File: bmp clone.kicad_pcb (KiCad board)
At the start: 2 copper layers, 56.5 x 29.8 mm, 46 parts, among them J1 Conn_02x10_Odd_Even, J3 Jumper_2_Open, P1 USB_C_Plug_USB2.0, Q1 BC846, U1 STM32F103RBTx, U2 USBLC6-2P6, U3 TXS0108EPW, U4 AMS1117-3.3, X1 8MHz

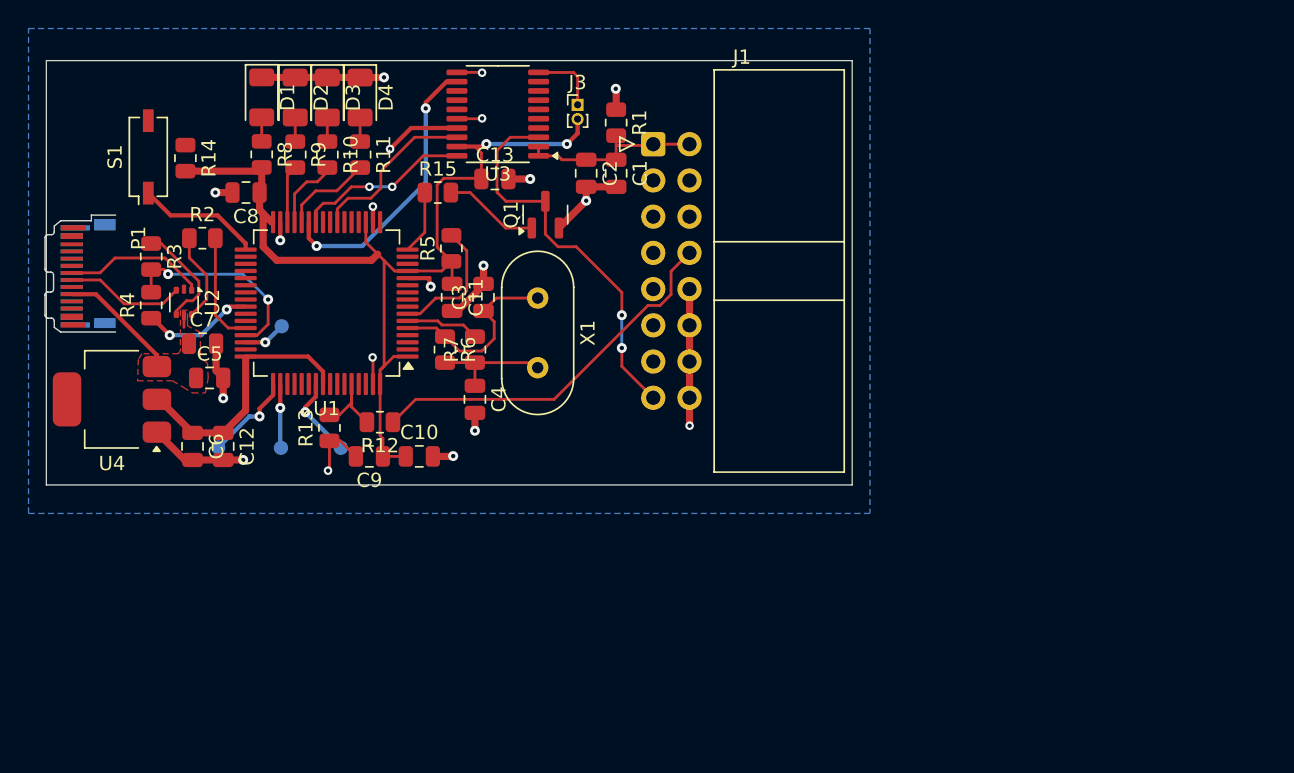
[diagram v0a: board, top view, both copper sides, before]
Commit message: pcb
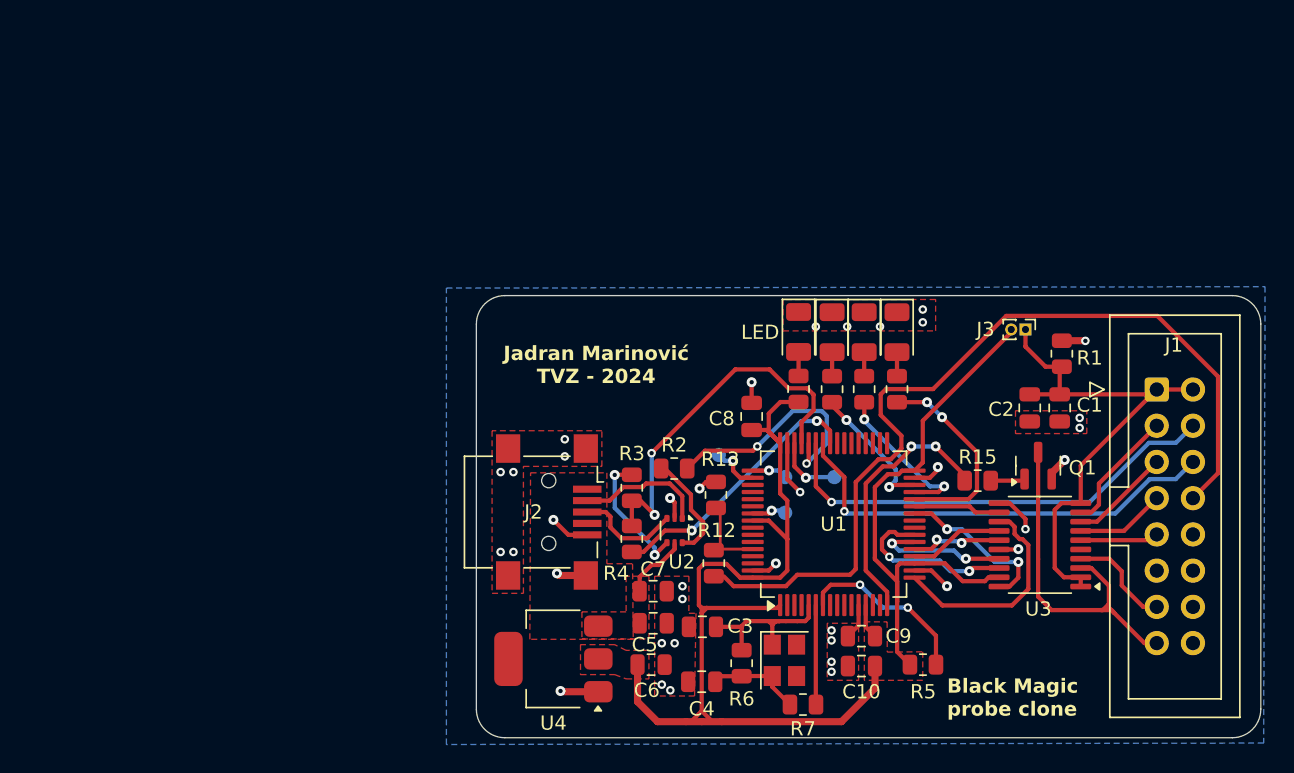
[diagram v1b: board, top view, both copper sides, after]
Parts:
- removed C11, C12, C13: 100n, Capacitor_SMD:C_0805_2012Metric
- removed P1: USB_C_Plug_USB2.0, Connector_USB:USB_C_Plug_JAE_DX07P024AJ1
- removed R14: 1k, Resistor_SMD:R_0805_2012Metric
- removed S1: SW_MEC_5G, Button_Switch_SMD:SW_DIP_SPSTx01_Slide_Copal_CHS-01A_W5.08mm_P1.27mm_JPin
- added J2: USB_B_Mini, Connector_USB:USB_Mini-B_Lumberg_2486_01_Horizontal, F.Cu at (117.5, 90.9)
- J1: footprint Connector_IDC:IDC-Header_2x08_P2.54mm_Horizontal -> Connector_IDC:IDC-Header_2x08_P2.54mm_Vertical
- X1: footprint Crystal:Crystal_HC49-4H_Vertical -> Crystal:Crystal_SMD_3225-4Pin_3.2x2.5mm
- moved U3 48.5 mm to (151.9, 93.2)
- moved R5 44.1 mm to (143.7, 101.6), turned to 0 degrees
- moved R15 42.9 mm to (147.6, 88.7)
- moved D2 41.1 mm to (137.3, 78.3)
- moved D3 41.1 mm to (139.6, 78.3)
- moved R10 41.1 mm to (139.6, 82.3)
- moved R9 41.1 mm to (137.3, 82.3)
- moved D4 41.1 mm to (141.9, 78.3)
- moved LED 41.1 mm to (135.0, 78.3)
- moved R8 41.1 mm to (135.0, 82.3)
- moved R11 41.1 mm to (141.9, 82.3)
- moved TP1 40.2 mm to (137.5, 88.5)
- moved TP2 39.8 mm to (134.1, 88.5)
- moved J1 39.3 mm to (160.1, 82.3)
- moved U1 38.8 mm to (137.4, 91.8), turned to 90 degrees
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- renumbered D1 to LED
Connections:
- U1 pad 33: Net-(U1-PB12) -> unconnected-(U1-PB12-Pad33)
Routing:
- net /BOOT_0: track 26.7 -> 61.7 mm
- net /U1RX: track 0.00 -> 32.1 mm, vias 0 -> 1
- net /U1TX: track 0.00 -> 31.4 mm, vias 0 -> 1
- net GND: track 60.6 -> 32.9 mm, vias 18 -> 37
- net +3.3V: track 89.9 -> 110.3 mm, vias 2 -> 0
- net Net-(J1-Pin_1): track 17.8 -> 36.9 mm
- net /xTDI: track 0.00 -> 15.4 mm
- net /xnSRST_OUT: track 4.50 -> 18.5 mm, vias 0 -> 2
- net /xnTRST: track 19.8 -> 6.10 mm, vias 2 -> 0
- net /USB_DP: track 14.3 -> 26.5 mm
- net /USB_PU: track 7.95 -> 18.9 mm
- net /USB_DM: track 7.90 -> 17.0 mm, vias 0 -> 2
- net Net-(U1-PB12): track 8.71 -> 0.00 mm
- net Net-(J1-Pin_3): track 0.00 -> 8.71 mm
- net /LED_0: track 6.39 -> 14.4 mm, vias 0 -> 2
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- added copper zone on F.Cu, net +3.3V
- added copper zone on F.Cu, net GND
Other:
- board size 56.5 x 29.8 mm -> 55 x 31 mm
- board text added: "Black Magic probe clone"
- board text added: "Jadran Marinović TVZ - 2024"
